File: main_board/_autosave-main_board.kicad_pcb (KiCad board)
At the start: 2 copper layers, 146 x 111.8 mm, 128 parts, among them J1 stepper 0, J10 24VDC output 5, J11 5VDC output 0, J12 5VDC output 1, J13 5VDC output 2, J14 5VDC output 3, J15 5VDC output 4, J16 5VDC output 5, J17 temperature measure 0, J18 temperature measure 1, J19 I2C, J2 stepper 1, J20 I2C, J21 I2C, J22 I2C, J23 hall measure 0, J24 weight measure 0, J25 light measure 0, J26 24VDC_in, J27 24VDC to 5VDC step down, J28 24VDC, J29 24VDC, J3 stepper 2, J30 24VDC, J31 5VDC, J32 5VDC, J33 5VDC, J34 hall measure 1, J35 reflective sensor 0, J36 24VDC, J37 24VDC, J38 24VDC, J39 5VDC, J4 stepper 3, J40 5VDC, J41 5VDC, J42 Conn_01x05_Male, J5 24VDC output 0, J6 24VDC output 1, J7 24VDC output 2, J8 24VDC output 3, J9 24VDC output 4, Q1 Q_NMOS_GDS, Q10 BS170, Q11 BS170, Q12 BS170, Q2 Q_NMOS_GDS, Q3 Q_NMOS_GDS, Q4 Q_NMOS_GDS, Q5 Q_NMOS_GDS, Q6 Q_NMOS_GDS, Q7 BS170, Q8 BS170, Q9 BS170, U1 ESP32-DEVKITC-32D, U2 PCA9685PW

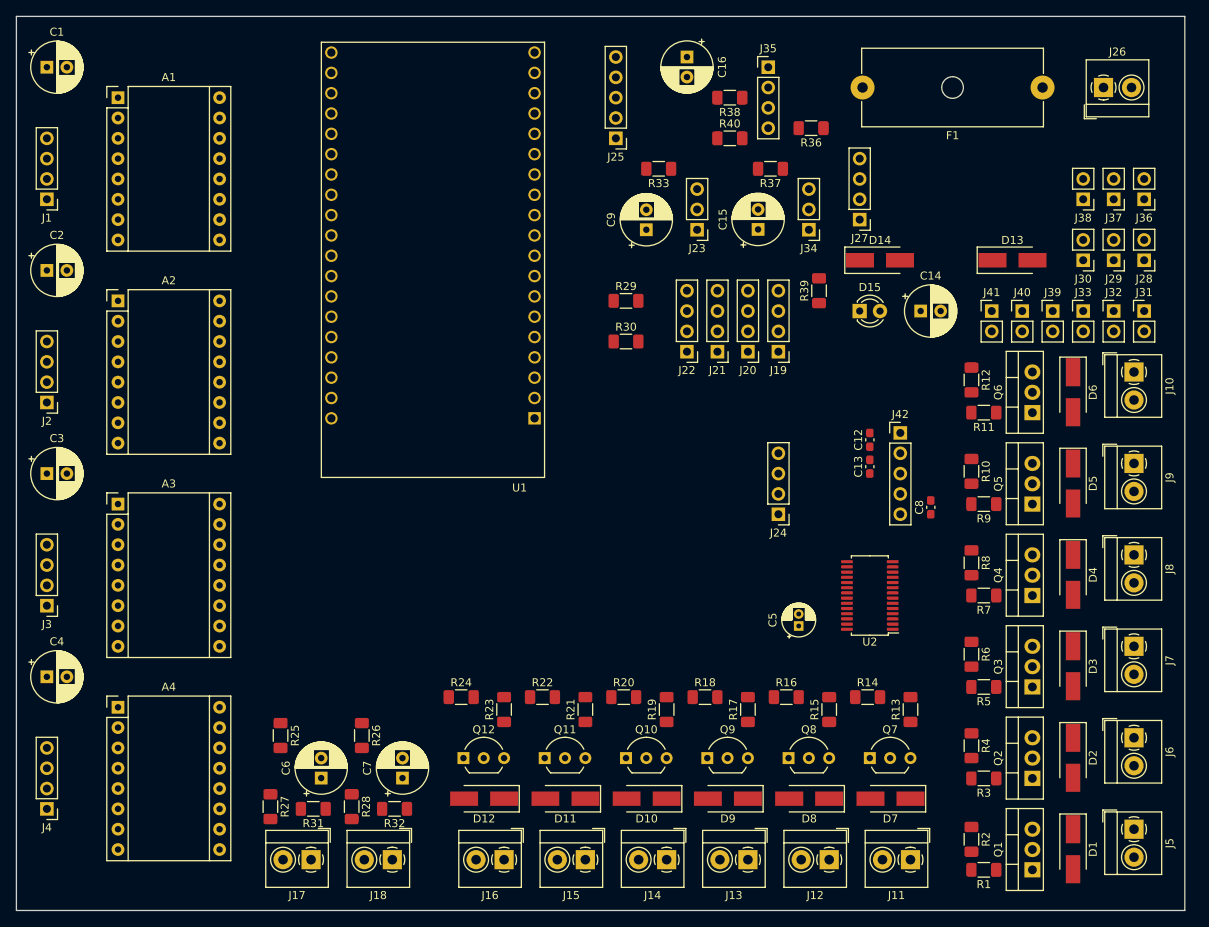
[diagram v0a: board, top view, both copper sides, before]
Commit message: routs added
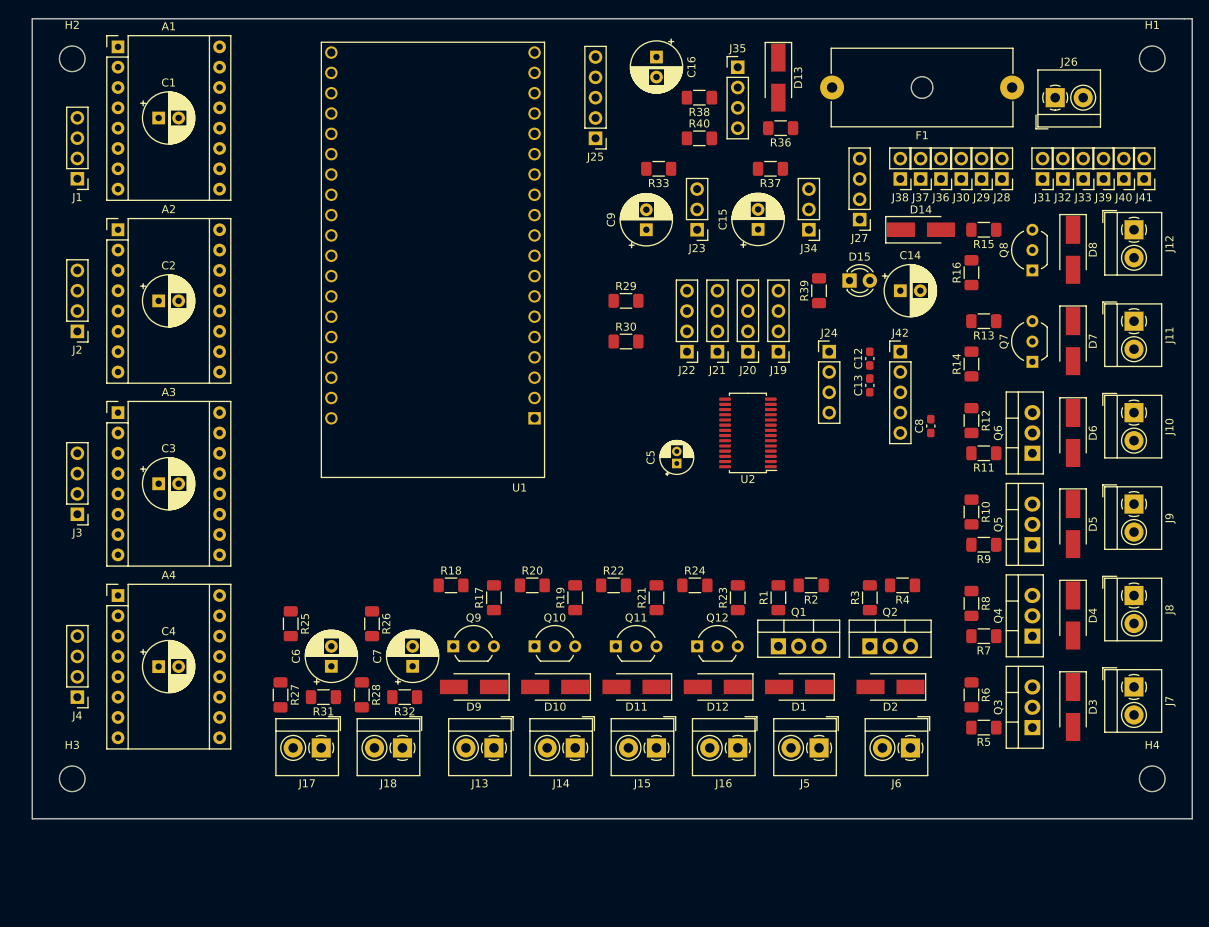
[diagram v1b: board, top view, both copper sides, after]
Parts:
- added H1: MountingHole, MountingHole:MountingHole_3.2mm_M3, F.Cu at (175.0, 18.0)
- added H2: MountingHole, MountingHole:MountingHole_3.2mm_M3, F.Cu at (40.0, 18.0)
- added H3: MountingHole, MountingHole:MountingHole_3.2mm_M3, F.Cu at (40.0, 108.0)
- added H4: MountingHole, MountingHole:MountingHole_3.2mm_M3, F.Cu at (175.0, 108.0)
- moved J12 87.5 mm to (172.7, 39.4), turned to 270 degrees
- moved D8 76.1 mm to (165.1, 41.9), turned to 270 degrees
- moved J11 72.9 mm to (172.7, 50.8), turned to 270 degrees
- moved Q8 68.2 mm to (160.0, 44.5), turned to 90 degrees
- moved R15 63.0 mm to (153.9, 39.4), turned to 180 degrees
- moved D7 61.6 mm to (165.1, 53.3), turned to 270 degrees
- moved R16 57.9 mm to (152.4, 44.7), turned to 90 degrees
- moved Q7 53.5 mm to (160.0, 55.9), turned to 90 degrees
- moved R13 49.4 mm to (153.9, 50.8), turned to 180 degrees
- moved R14 43.6 mm to (152.4, 56.2), turned to 90 degrees
- moved R1 42.6 mm to (128.3, 85.4), turned to 90 degrees
- moved Q1 42.3 mm to (128.3, 91.4), turned to 0 degrees
- moved J5 40.7 mm to (133.3, 104.1), turned to 180 degrees
- moved D1 39.8 mm to (130.8, 96.5), turned to 180 degrees
- moved R2 37.5 mm to (132.4, 83.8), turned to 180 degrees
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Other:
- board size 146 x 111.8 mm -> 145 x 100 mm
